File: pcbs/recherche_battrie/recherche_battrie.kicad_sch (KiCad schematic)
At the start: 5 parts, among them Q1 Q_Dual_NMOS_S1G1D2S2G2D1, U1 TP4056-42-ESOP8, U2 DW01A, U3 ME6211C33M5, U4 TPL5110

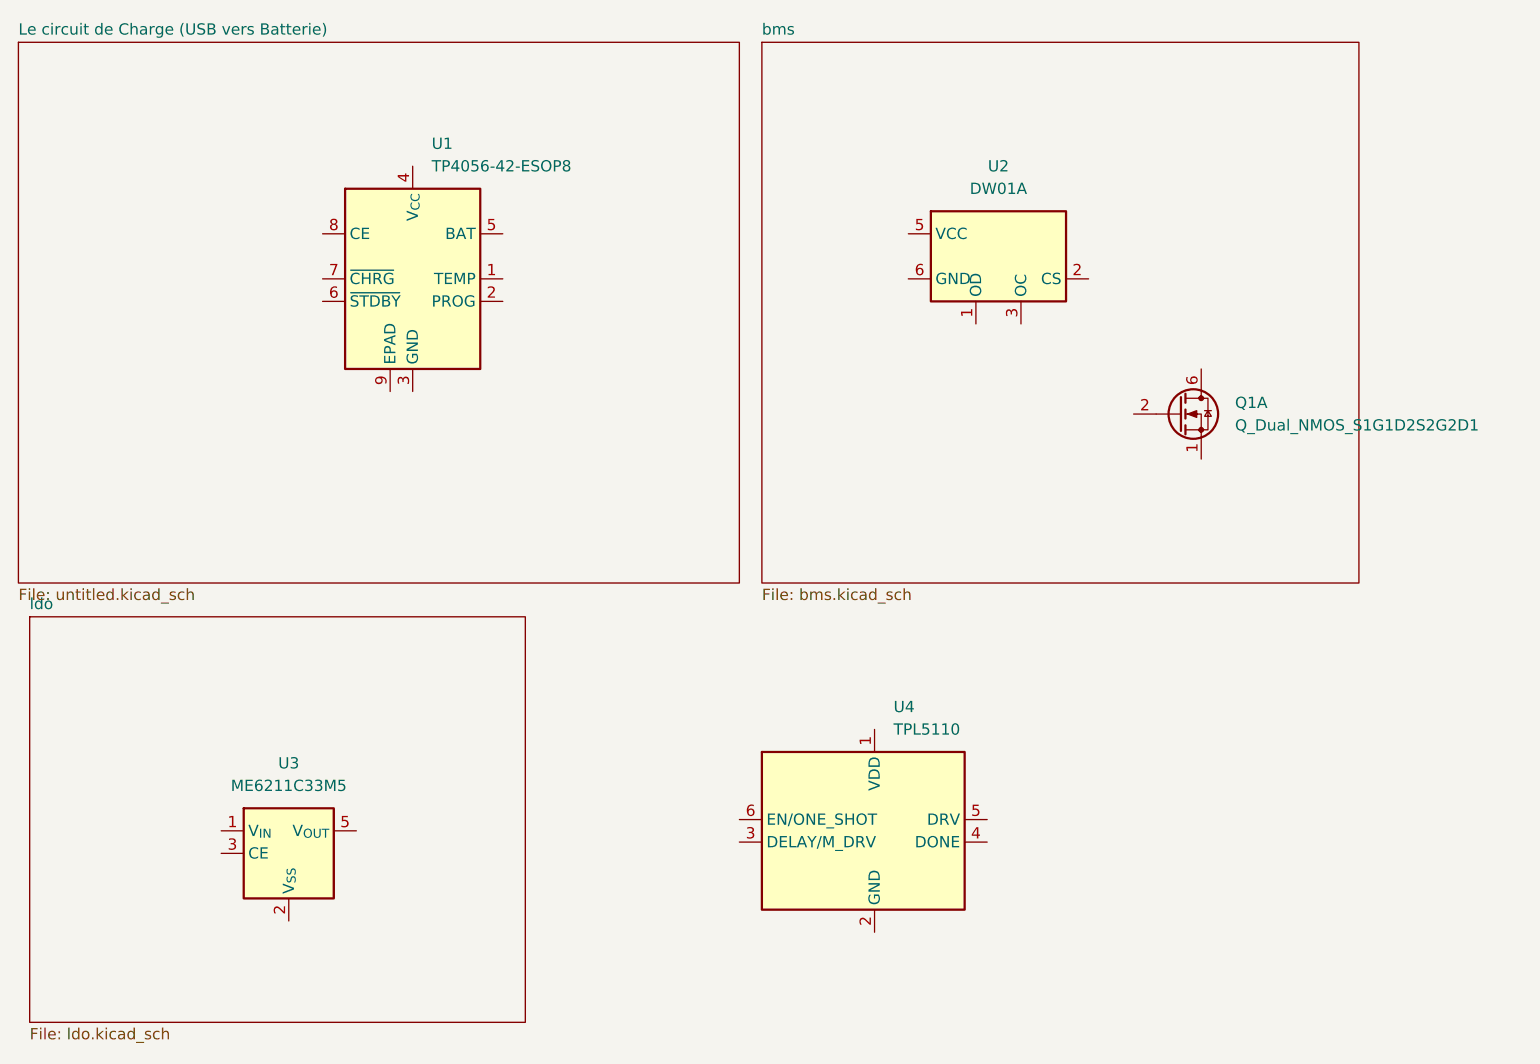
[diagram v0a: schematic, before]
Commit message: pcb recherche routage pas fini
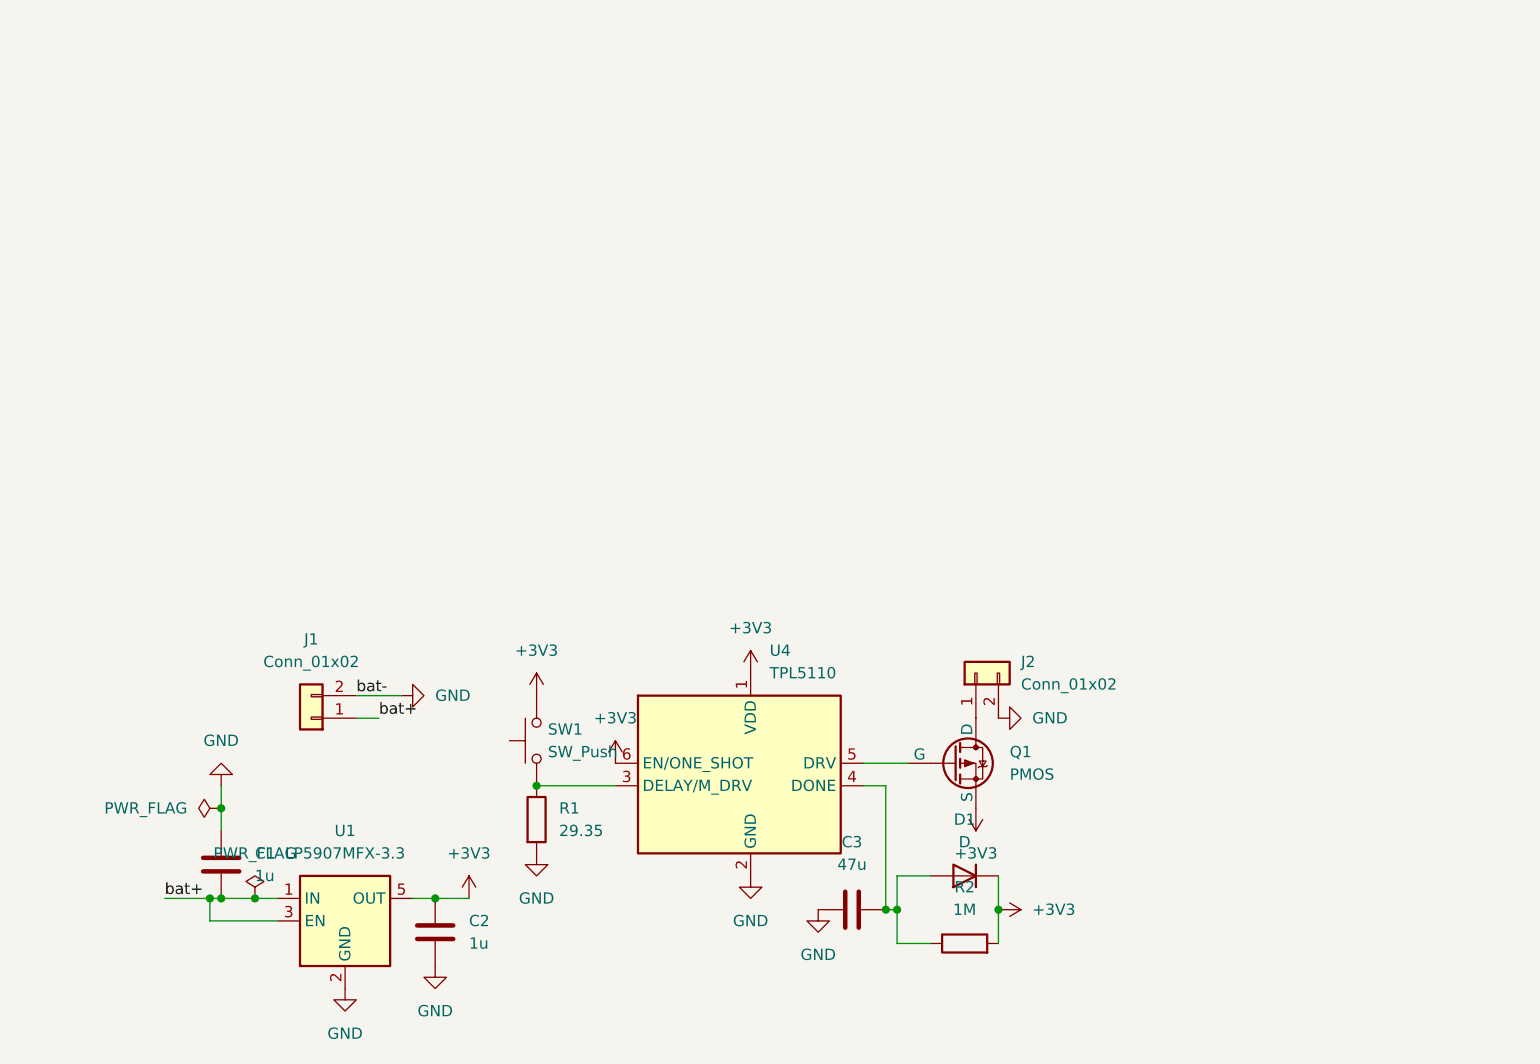
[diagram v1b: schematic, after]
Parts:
- removed Q1: Q_Dual_NMOS_S1G1D2S2G2D1, symbol Transistor_FET:Q_Dual_NMOS_S1G1D2S2G2D1
- removed U1: TP4056-42-ESOP8, Package_SO:SOIC-8-1EP_3.9x4.9mm_P1.27mm_EP2.41x3.3mm_ThermalVias, symbol Battery_Management:TP4056-42-ESOP8
- removed U2: DW01A, Package_TO_SOT_SMD:SOT-23-6, symbol Battery_Management:DW01A
- removed U3: ME6211C33M5, Package_TO_SOT_SMD:SOT-23-5, symbol Regulator_Linear:ME6211C33M5
- added C1, C2: 1u, Capacitor_SMD:C_0805_2012Metric, symbol Device:C
- added C3: 47u, Capacitor_SMD:C_1206_3216Metric, symbol Device:C
- added D1: D, Diode_SMD:D_SOD-123, symbol Device:D
- added J1, J2: Conn_01x02, Connector_PinHeader_2.54mm:PinHeader_1x02_P2.54mm_Vertical, symbol Connector_Generic:Conn_01x02
- added Q1: PMOS, Package_TO_SOT_SMD:SOT-23, symbol Simulation_SPICE:PMOS
- added R1: 29.35, Resistor_SMD:R_0805_2012Metric, symbol Device:R
- added R2: 1M, Resistor_SMD:R_0805_2012Metric, symbol Device:R
- added SW1: SW_Push, Button_Switch_SMD:SW_SPST_B3U-1000P, symbol Switch:SW_Push
- added U1: LP5907MFX-3.3, Package_TO_SOT_SMD:SOT-23-5, symbol Regulator_Linear:LP5907MFX-3.3
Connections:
- net +3V3: now reaches U4.1 (VDD)
- net +3V3: now also U4.6 (EN/ONE_SHOT), C2.1, D1.1 (K), Q1.3 (S), R2.2, SW1.2, U1.5 (OUT)
- net GND: now reaches U4.2 (GND)
- net GND: now also C1.1, C2.2, C3.1, J1.2 (Pin_2), J2.2 (Pin_2), R1.2, U1.2 (GND)
- net at U4.3 (DELAY/M_DRV): now also R1.1, SW1.1
- net at U4.4 (DONE): now also C3.2, D1.2 (A), R2.1
- net at U4.5 (DRV): now also Q1.2 (G)
- new net: J2.1 (Pin_1), Q1.1 (D)
- new net bat+: C1.2, J1.1 (Pin_1), U1.1 (IN), U1.3 (EN)
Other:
- removed sheet Le circuit de Charge (USB vers Batterie)
- removed sheet bms
- removed sheet ldo
- moved on the sheet: U4
